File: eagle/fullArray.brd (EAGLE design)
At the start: 43 x 72 mm, 119 parts

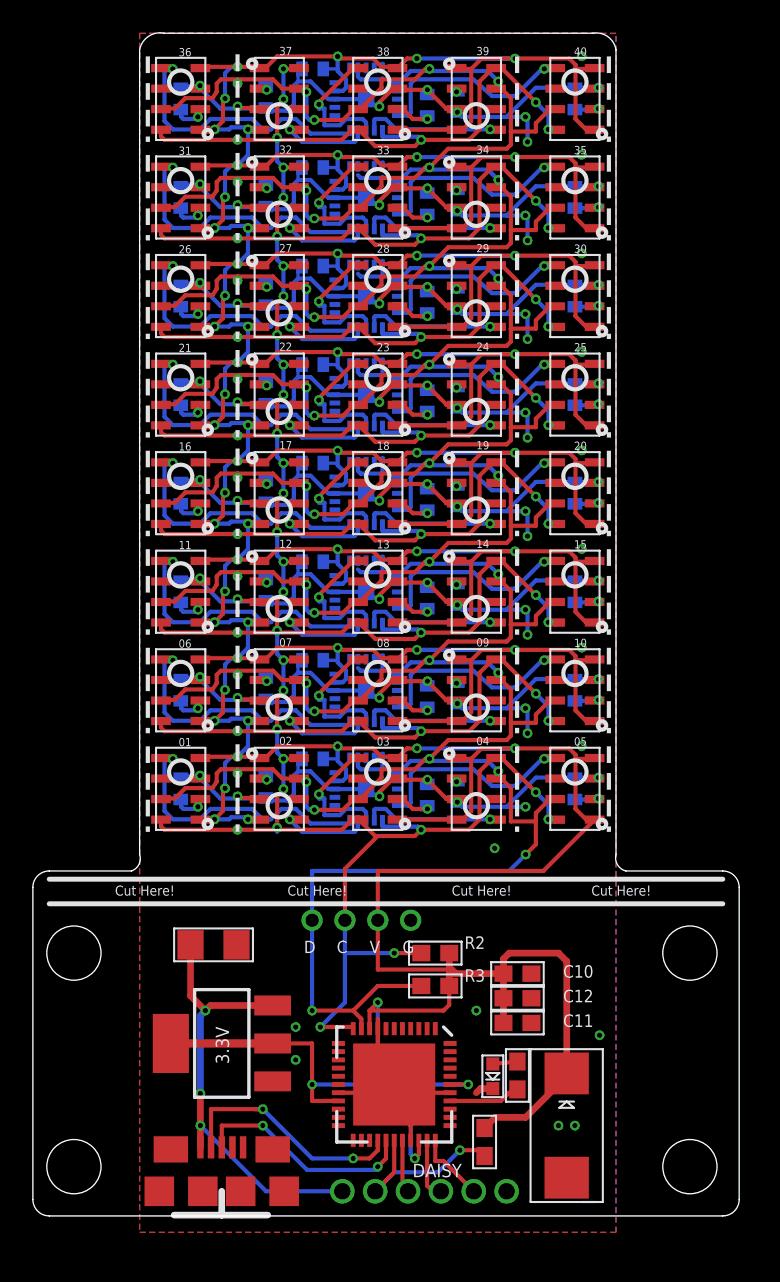
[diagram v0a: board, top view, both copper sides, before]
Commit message: center, center, and recenter...
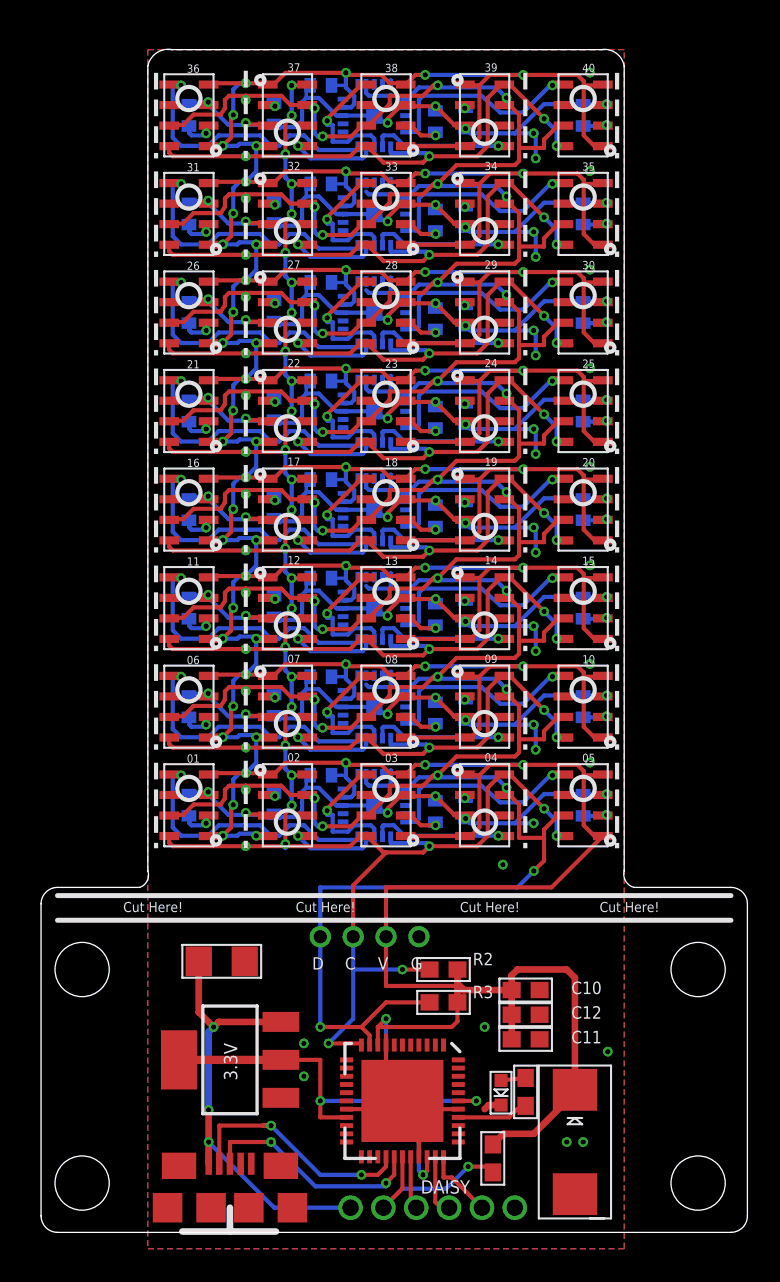
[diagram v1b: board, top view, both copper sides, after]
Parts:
- moved 01 1.12 mm to (2.50, 26.0)
- moved 02 1.12 mm to (8.50, 26.0)
- moved 03 1.12 mm to (14.5, 26.0)
- moved 04 1.12 mm to (20.5, 26.0)
- moved 05 1.12 mm to (26.5, 26.0)
- moved 06 1.12 mm to (2.50, 32.0)
- moved 07 1.12 mm to (8.50, 32.0)
- moved 08 1.12 mm to (14.5, 32.0)
- moved 09 1.12 mm to (20.5, 32.0)
- moved 10 1.12 mm to (26.5, 32.0)
- moved 11 1.12 mm to (2.50, 38.0)
- moved 12 1.12 mm to (8.50, 38.0)
- moved 13 1.12 mm to (14.5, 38.0)
- moved 14 1.12 mm to (20.5, 38.0)
- moved 15 1.12 mm to (26.5, 38.0)
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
